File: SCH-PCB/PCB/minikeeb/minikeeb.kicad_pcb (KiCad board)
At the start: 2 copper layers, 99.8 x 91 mm, 93 parts, among them J1 OLED, SW1 SW_PUSH-Lily58-cache, SW10 SW_PUSH-Lily58-cache, SW11 SW_PUSH-Lily58-cache, SW12 SW_PUSH-Lily58-cache, SW13 SW_PUSH-Lily58-cache, SW14 SW_PUSH-Lily58-cache, SW15 SW_PUSH-Lily58-cache, SW16 SW_PUSH-Lily58-cache, SW17 SW_PUSH-Lily58-cache, SW18 SW_PUSH-Lily58-cache, SW19 SW_PUSH-Lily58-cache, SW2 SW_PUSH-Lily58-cache, SW20 Rotary_Encoder_Switch-Device, SW3 SW_PUSH-Lily58-cache, SW4 SW_PUSH-Lily58-cache, SW5 SW_PUSH-Lily58-cache, SW6 SW_PUSH-Lily58-cache, SW7 SW_PUSH-Lily58-cache, SW8 SW_PUSH-Lily58-cache, SW9 SW_PUSH-Lily58-cache, U1 ProMicro_2-Lily58-cache, U2 TRRS

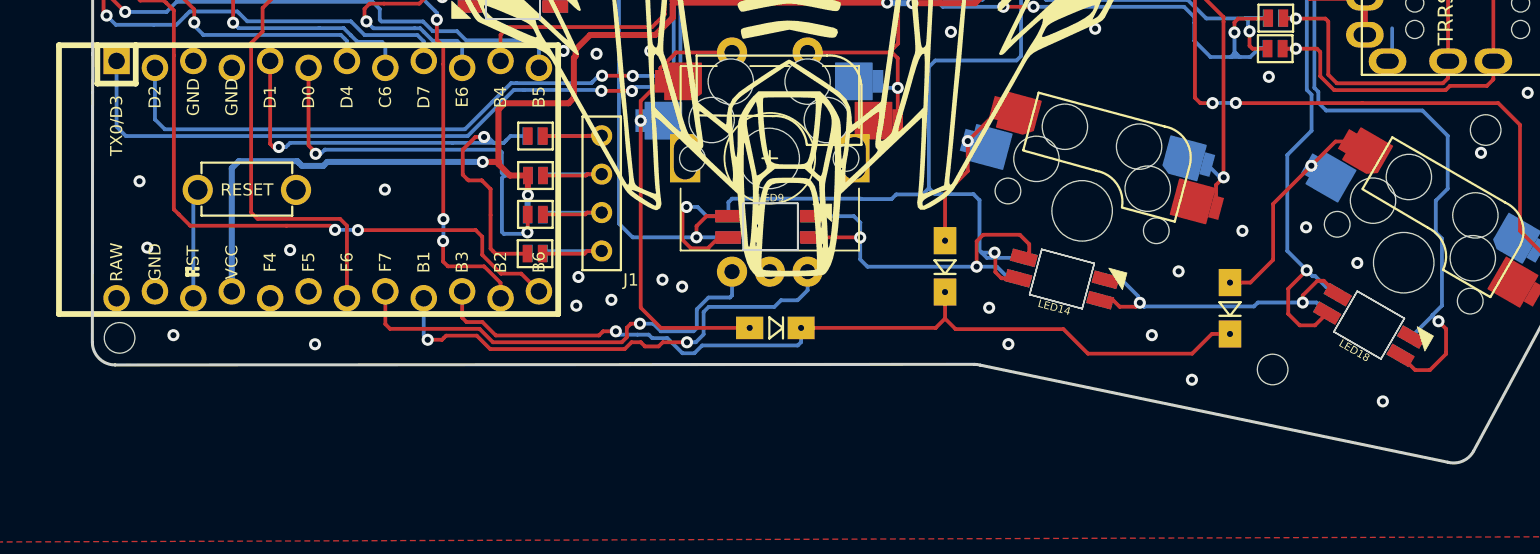
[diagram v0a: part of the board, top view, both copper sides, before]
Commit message: FEAT: update pcb
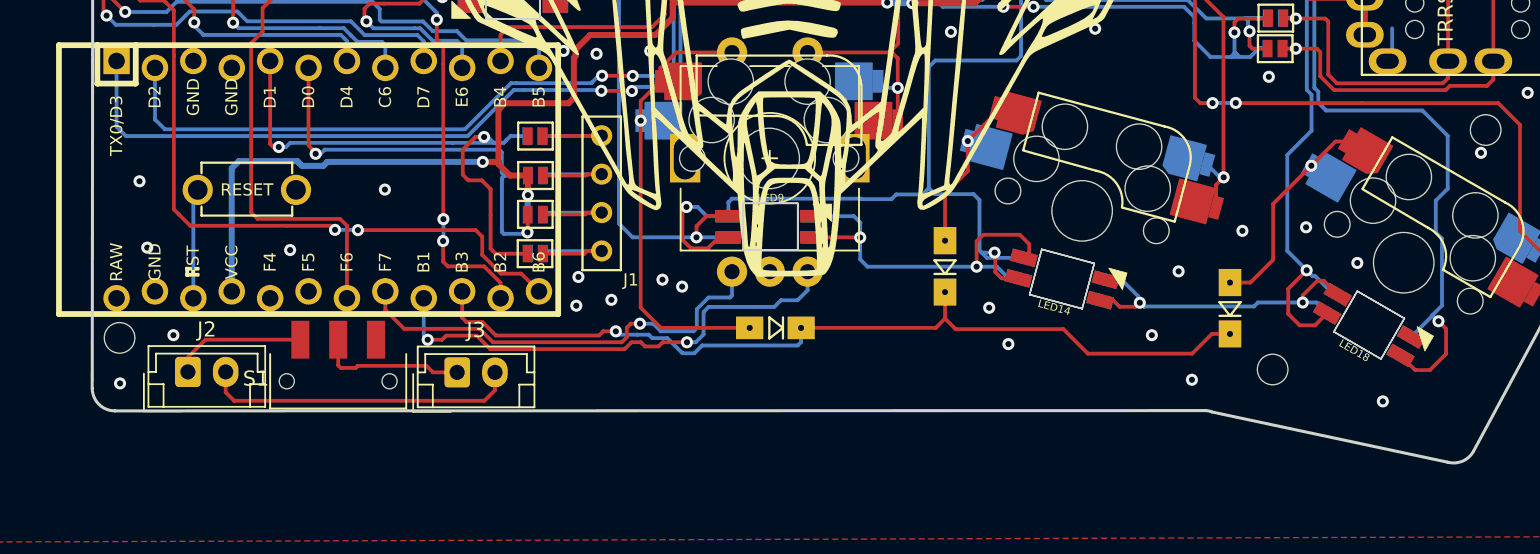
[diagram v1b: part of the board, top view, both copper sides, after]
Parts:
- added J2: Conn_01x02_Pin, Connector_JST:JST_EH_B2B-EH-A_1x02_P2.50mm_Vertical, F.Cu at (36.4, 151.9)
- added J3: Conn_01x02_Pin, Connector_JST:JST_EH_B2B-EH-A_1x02_P2.50mm_Vertical, F.Cu at (54.2, 152.0)
- added S1: JS102011SAQN, other:SW_JS102011SAQN, F.Cu at (46.4, 152.6)
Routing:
- net Net-(J2-Pin_2): track 0.00 -> 20.9 mm
- net Net-(J3-Pin_1): track 0.00 -> 9.87 mm
- net Net-(J2-Pin_1): track 0.00 -> 8.89 mm
- net ench_a: track 30.0 -> 29.4 mm
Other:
- board size 99.8 x 91 mm -> 99.9 x 91 mm
